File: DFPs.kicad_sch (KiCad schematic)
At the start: 18 parts

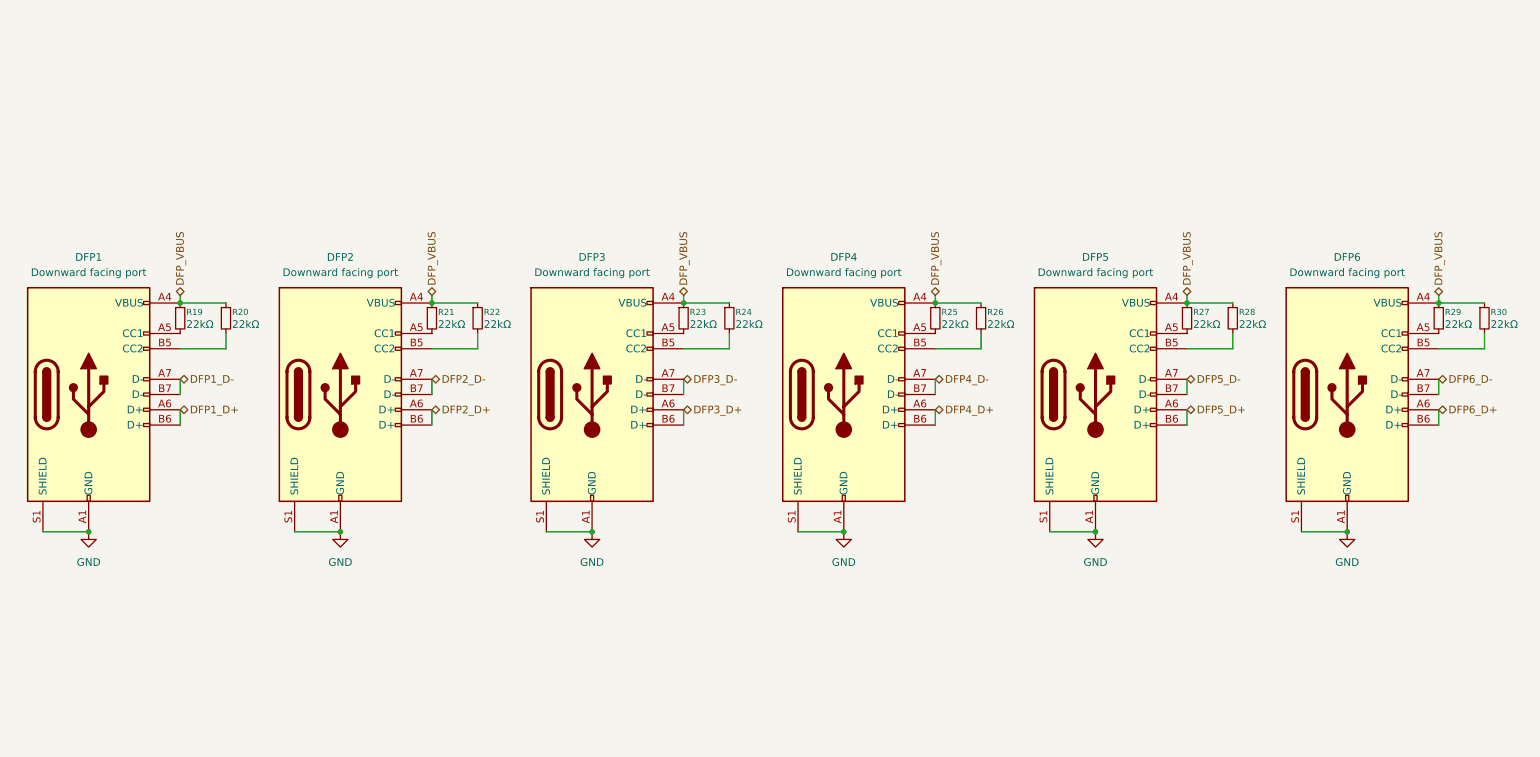
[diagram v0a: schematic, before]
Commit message: Update DFPs
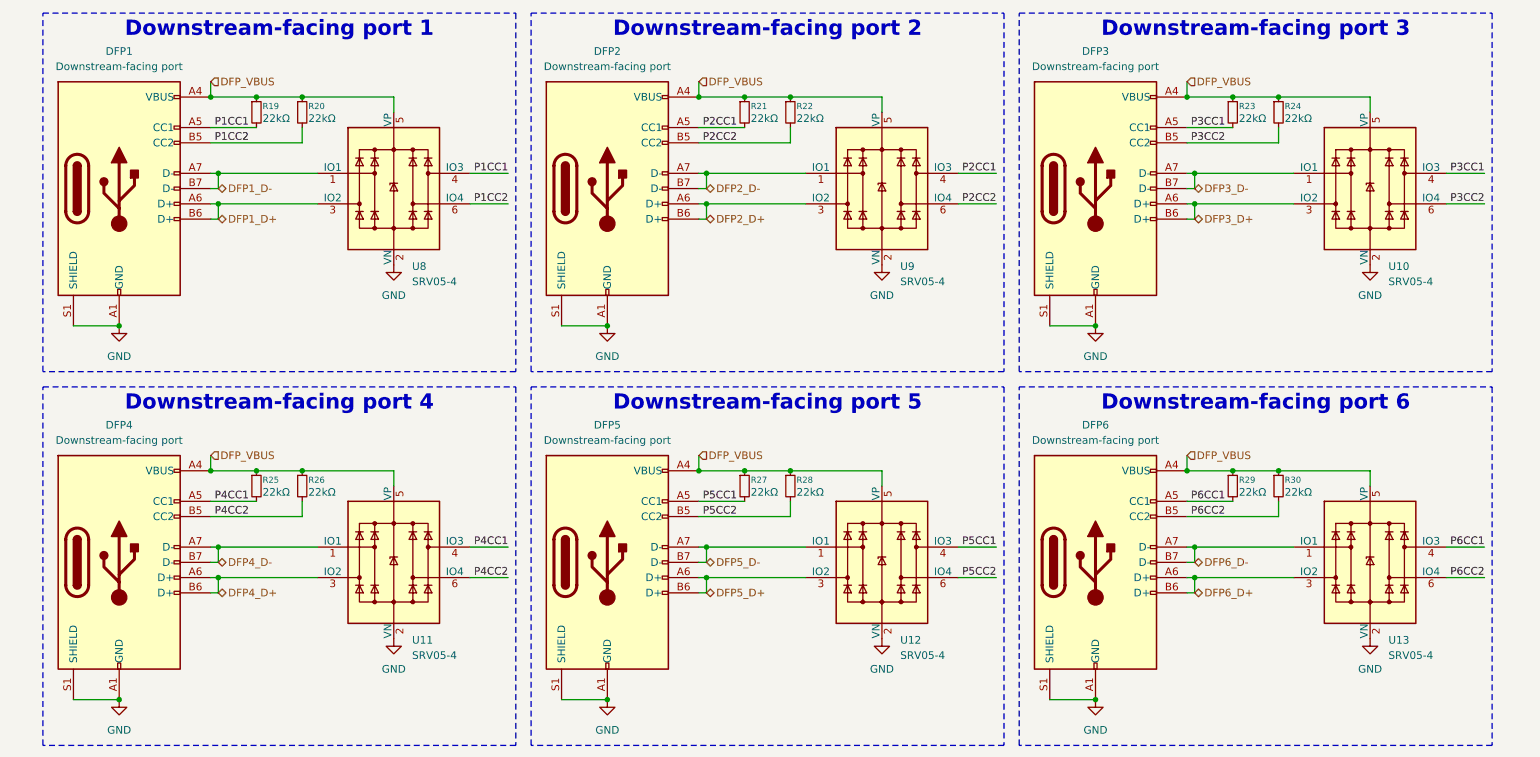
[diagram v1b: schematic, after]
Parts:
- added U10, U11, U12, U13, U8, U9: SRV05-4, Package_TO_SOT_SMD:SOT-23-6, symbol Power_Protection:SRV05-4
- DFP1, DFP2, DFP3, DFP4, DFP5, DFP6: value Downward facing port -> Downstream-facing port
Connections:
- net DFP1_D+: now also U8.3 (IO2)
- net DFP1_D-: now also U8.1 (IO1)
- net DFP2_D+: now also U9.3 (IO2)
- net DFP2_D-: now also U9.1 (IO1)
- net DFP3_D+: now also U10.3 (IO2)
- net DFP3_D-: now also U10.1 (IO1)
- net DFP4_D+: now also U11.3 (IO2)
- net DFP4_D-: now also U11.1 (IO1)
- net DFP5_D+: now also U12.3 (IO2)
- net DFP5_D-: now also U12.1 (IO1)
- net DFP6_D+: now also U13.3 (IO2)
- net DFP6_D-: now also U13.1 (IO1)
- net DFP_VBUS: now also U10.5 (VP), U11.5 (VP), U12.5 (VP), U13.5 (VP), U8.5 (VP), U9.5 (VP)
- net GND: now also U10.2 (VN), U11.2 (VN), U12.2 (VN), U13.2 (VN), U8.2 (VN), U9.2 (VN)
- net P5CC1: now reaches DFP5.A5 (CC1), R27.2
- net P5CC1: now also U12.4 (IO3)
- net P5CC2: now reaches DFP5.B5 (CC2), R28.2
- net P5CC2: now also U12.6 (IO4)
- net P1CC1: now reaches DFP1.A5 (CC1), R19.2
- net P1CC1: now also U8.4 (IO3)
- net P3CC2: now reaches DFP3.B5 (CC2), R24.2
- net P3CC2: now also U10.6 (IO4)
- net P4CC1: now reaches DFP4.A5 (CC1), R25.2
- net P4CC1: now also U11.4 (IO3)
- net P4CC2: now reaches DFP4.B5 (CC2), R26.2
- net P4CC2: now also U11.6 (IO4)
- net P2CC2: now reaches DFP2.B5 (CC2), R22.2
- net P2CC2: now also U9.6 (IO4)
- net P6CC1: now reaches DFP6.A5 (CC1), R29.2
- net P6CC1: now also U13.4 (IO3)
- net P6CC2: now reaches DFP6.B5 (CC2), R30.2
- net P6CC2: now also U13.6 (IO4)
- net P3CC1: now reaches DFP3.A5 (CC1), R23.2
- net P3CC1: now also U10.4 (IO3)
- net P1CC2: now reaches DFP1.B5 (CC2), R20.2
- net P1CC2: now also U8.6 (IO4)
- net P2CC1: now reaches DFP2.A5 (CC1), R21.2
- net P2CC1: now also U9.4 (IO3)
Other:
- moved on the sheet: DFP1, R19, R20

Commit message: footprints
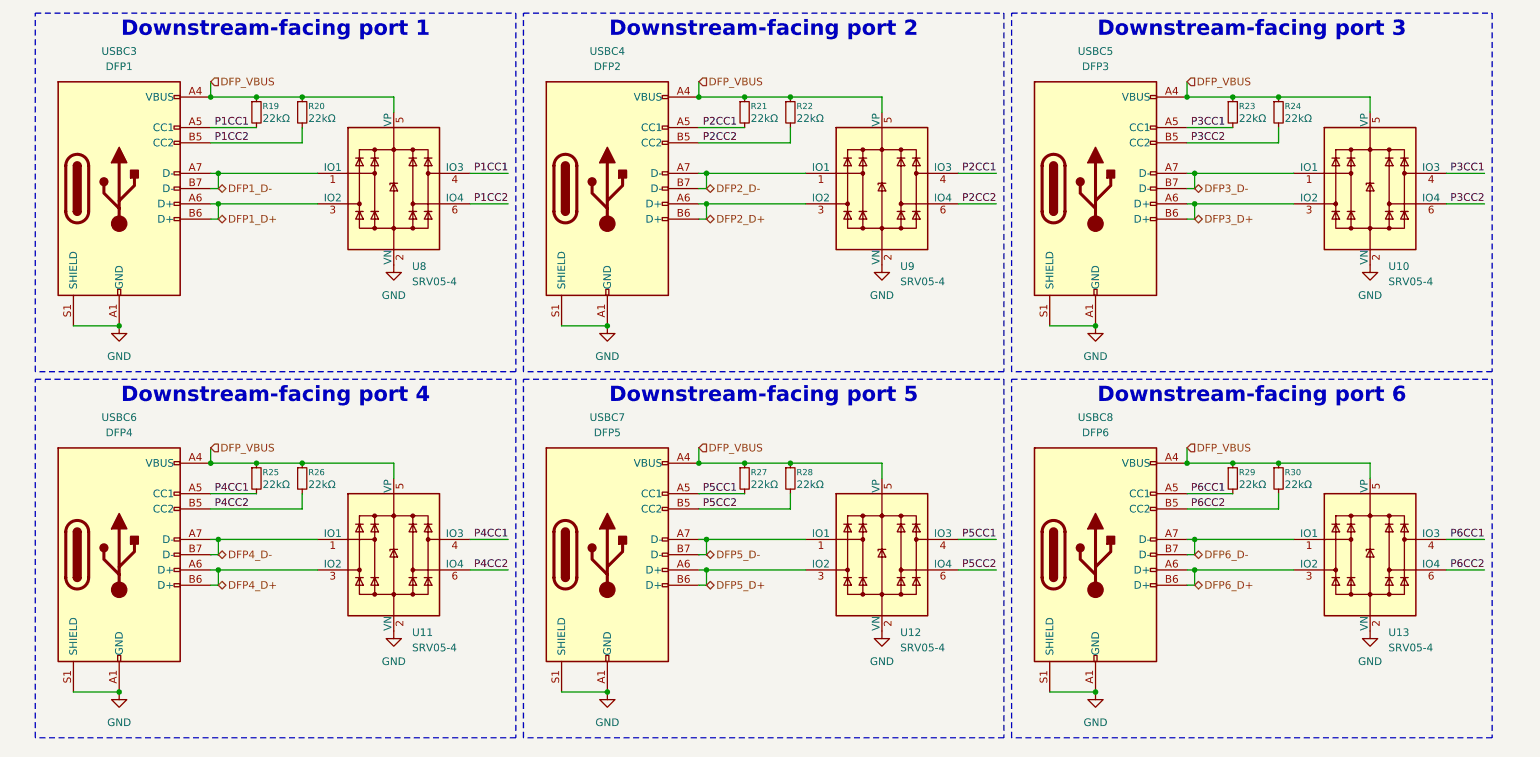
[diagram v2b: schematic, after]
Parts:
- R19, R20, R21, R22, R23, R24, R25, R26, R27, R28, R29, R30: footprint (none) -> Resistor_SMD:R_0603_1608Metric
- USBC3: renamed from DFP1; value Downstream-facing port -> DFP1
- USBC4: renamed from DFP2; value Downstream-facing port -> DFP2
- USBC5: renamed from DFP3; value Downstream-facing port -> DFP3
- USBC6: renamed from DFP4; value Downstream-facing port -> DFP4
- USBC7: renamed from DFP5; value Downstream-facing port -> DFP5
- USBC8: renamed from DFP6; value Downstream-facing port -> DFP6
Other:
- moved on the sheet: R25, R26, R27, R28, R29, R30, U11, U12, U13, USBC6, USBC7, USBC8
